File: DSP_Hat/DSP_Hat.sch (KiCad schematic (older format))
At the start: 30 parts, among them P1 Conn_02x20_Odd_Even

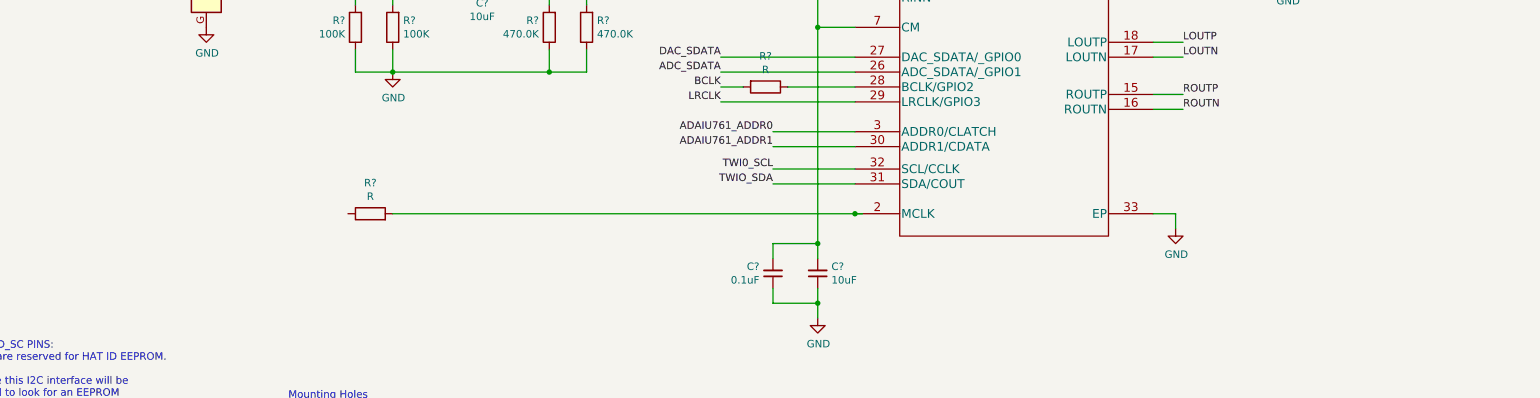
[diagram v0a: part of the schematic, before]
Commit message: added osc
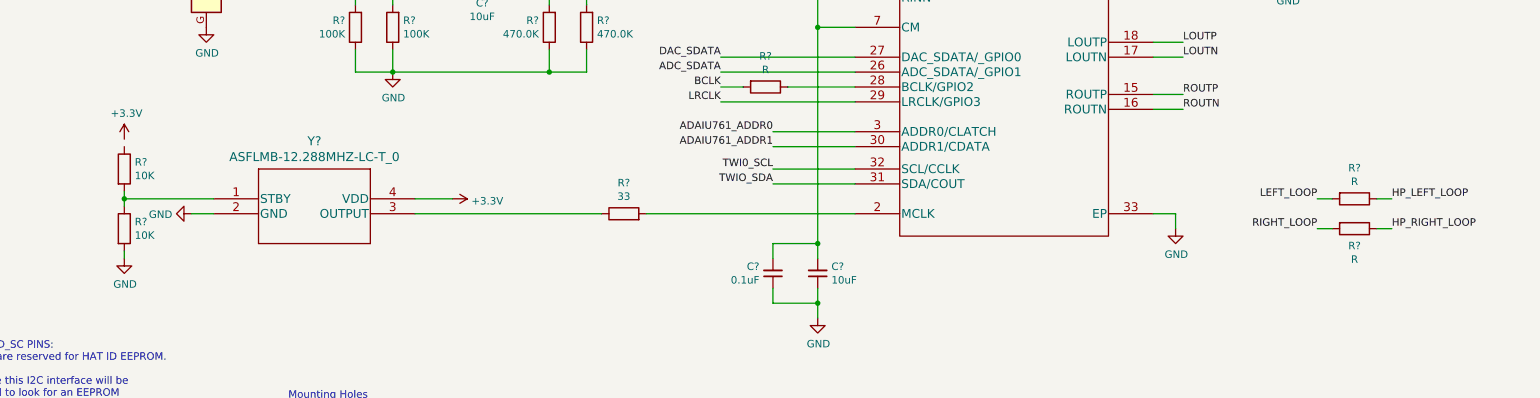
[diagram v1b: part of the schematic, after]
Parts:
- added R? (x2): R, symbol Device:R
- added R? (x2): 10K, symbol Device:R
- added Y?: ASFLMB-12.288MHZ-LC-T_0, ASFLMB_Series, symbol 2019-04-10_00-18-11:ASFLMB-12.288MHZ-LC-T_0
- R?: value R -> 33
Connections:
- net +3V3: now also Y?.4 (VDD)
- net GND: now also R?.2, Y?.2 (GND)
- net HP_LEFT_LOOP: now also R?.1
- net HP_RIGHT_LOOP: now also R?.1
- net LEFT_LOOP: now also R?.2
- net RIGHT_LOOP: now also R?.2
- net at R?.1: now also Y?.3 (OUTPUT)
- new net: R?.1, R?.2, Y?.1 (STBY)
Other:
- moved on the sheet: R?
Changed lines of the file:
@@
 	4150 4050 5000 4050
 Connection ~ 5000 4050
-Wire Wire Line
-	6850 5800 6800 5800
-Connection ~ 6800 5800
-Wire Wire Line
-	6800 5800 3700 5800
 $Comp
 L Device:R R?
 U 1 1 5CC86ACB
-P 3550 5800
-F 0 "R?" V 3757 5800 50  0000 C CNN
-F 1 "R" V 3666 5800 50  0000 C CNN
-F 2 "" V 3480 5800 50  0001 C CNN
-F 3 "~" H 3550 5800 50  0001 C CNN
-	1    3550 5800
+P 5250 5800
+F 0 "R?" V 5457 5800 50  0000 C CNN
+F 1 "33" V 5366 5800 50  0000 C CNN
+F 2 "" V 5180 5800 50  0001 C CNN
+F 3 "~" H 5250 5800 50  0001 C CNN
+	1    5250 5800
 	0    -1   -1   0
 $EndComp
@@
 	6550 6400 6550 6300
 Connection ~ 6550 6400
+$Comp
+L Device:R R?
+U 1 1 5CAE0EC7
+P 10150 5700
+F 0 "R?" V 9943 5700 50  0000 C CNN
+F 1 "R" V 10034 5700 50  0000 C CNN
+F 2 "" V 10080 5700 50  0001 C CNN
+F 3 "~" H 10150 5700 50  0001 C CNN
+	1    10150 5700
+	0    1    1    0
+$EndComp
+$Comp
+L Device:R R?
+U 1 1 5CAE0FB9
+P 10150 5900
+F 0 "R?" V 10265 5900 50  0000 C CNN
+F 1 "R" V 10356 5900 50  0000 C CNN
+F 2 "" V 10080 5900 50  0001 C CNN
+F 3 "~" H 10150 5900 50  0001 C CNN
+	1    10150 5900
+	0    1    1    0
+$EndComp
+Wire Wire Line
+	10300 5700 10400 5700
+Text Label 10400 5700 0    50   ~ 0
+HP_LEFT_LOOP
+Text Label 10400 5900 0    50   ~ 0
+HP_RIGHT_LOOP
+Wire Wire Line
+	10300 5900 10400 5900
+Wire Wire Line
+	10000 5700 9900 5700
+Wire Wire Line
+	10000 5900 9900 5900
+Text Label 9900 5700 2    50   ~ 0
+LEFT_LOOP
+Text Label 9900 5900 2    50   ~ 0
+RIGHT_LOOP
+$Comp
+L 2019-04-10_00-18-11:ASFLMB-12.288MHZ-LC-T_0 Y?
+U 1 1 5CAFC494
+P 2500 5700
+F 0 "Y?" H 3175 6087 60  0000 C CNN
+F 1 "ASFLMB-12.288MHZ-LC-T_0" H 3175 5981 60  0000 C CNN
+F 2 "ASFLMB_Series" H 3150 5950 60  0001 C CNN
+F 3 "" H 2500 5700 60  0000 C CNN
+	1    2500 5700
+	1    0    0    -1
+$EndComp
+Wire Wire Line
+	6800 5800 5400 5800
+Wire Wire Line
+	3850 5800 5100 5800
+$Comp
+L power:+3.3V #PWR?
+U 1 1 5CB3DF76
+P 4100 5700
+F 0 "#PWR?" H 4100 5550 50  0001 C CNN
+F 1 "+3.3V" V 4115 5828 50  0000 L CNN
+F 2 "" H 4100 5700 50  0001 C CNN
+F 3 "" H 4100 5700 50  0001 C CNN
+	1    4100 5700
+	0    1    1    0
+$EndComp
+Wire Wire Line
+	3850 5700 4100 5700
+$Comp
+L power:GND #PWR?
+U 1 1 5CB462D9
+P 2350 5800
+F 0 "#PWR?" H 2350 5550 50  0001 C CNN
+F 1 "GND" V 2355 5672 50  0000 R CNN
+F 2 "" H 2350 5800 50  0001 C CNN
+F 3 "" H 2350 5800 50  0001 C CNN
+	1    2350 5800
+	0    1    1    0
+$EndComp
+Wire Wire Line
+	2350 5800 2500 5800
+Wire Wire Line
+	2500 5700 1900 5700
+$Comp
+L power:GND #PWR?
+U 1 1 5CB5FE44
+P 1900 6100
+F 0 "#PWR?" H 1900 5850 50  0001 C CNN
+F 1 "GND" H 1905 5927 50  0000 C CNN
+F 2 "" H 1900 6100 50  0001 C CNN
+F 3 "" H 1900 6100 50  0001 C CNN
+	1    1900 6100
+	1    0    0    -1
+$EndComp
+$Comp
+L power:+3.3V #PWR?
+U 1 1 5CB5FED0
+P 1900 5300
+F 0 "#PWR?" H 1900 5150 50  0001 C CNN
+F 1 "+3.3V" H 1915 5473 50  0000 C CNN
+F 2 "" H 1900 5300 50  0001 C CNN
+F 3 "" H 1900 5300 50  0001 C CNN
+	1    1900 5300
+	1    0    0    -1
+$EndComp
+$Comp
+L Device:R R?
+U 1 1 5CB5FF6A
+P 1900 5500
+F 0 "R?" H 1970 5546 50  0000 L CNN
+F 1 "10K" H 1970 5455 50  0000 L CNN
+F 2 "" V 1830 5500 50  0001 C CNN
+F 3 "~" H 1900 5500 50  0001 C CNN
+	1    1900 5500
+	1    0    0    -1
+$EndComp
+$Comp
+L Device:R R?
+U 1 1 5CB6005E
+P 1900 5900
+F 0 "R?" H 1970 5946 50  0000 L CNN
+F 1 "10K" H 1970 5855 50  0000 L CNN
+F 2 "" V 1830 5900 50  0001 C CNN
+F 3 "~" H 1900 5900 50  0001 C CNN
+	1    1900 5900
+	1    0    0    -1
+$EndComp
+Wire Wire Line
+	1900 5700 1900 5650
+Wire Wire Line
+	1900 5700 1900 5750
+Connection ~ 1900 5700
+Wire Wire Line
+	1900 6050 1900 6100
 $EndSCHEMATC
